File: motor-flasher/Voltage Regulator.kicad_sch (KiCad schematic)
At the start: 3 parts, among them U3 LD1117S33TR

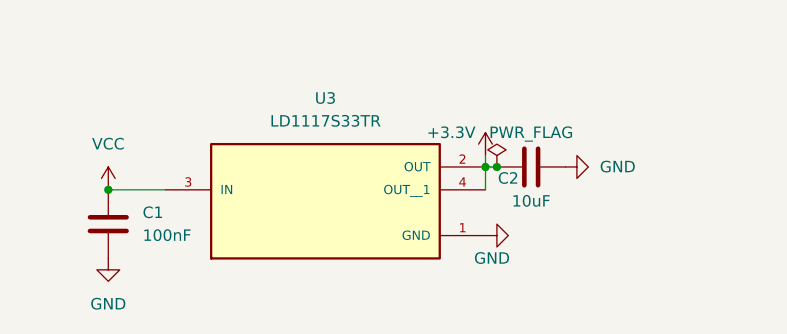
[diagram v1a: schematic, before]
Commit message: Beginning Layout Process
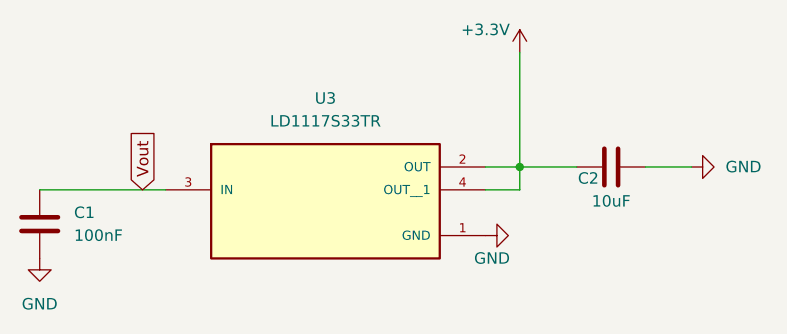
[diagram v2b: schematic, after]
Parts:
- U3: footprint revparts2:SOT230P700X180-4N -> Motor-Flasher:SOT230P700X180-4N
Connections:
- net VCC renamed Vout
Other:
- moved on the sheet: C1, C2
